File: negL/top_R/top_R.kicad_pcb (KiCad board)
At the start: 2 copper layers, 133.3 x 115.9 mm, 37 parts

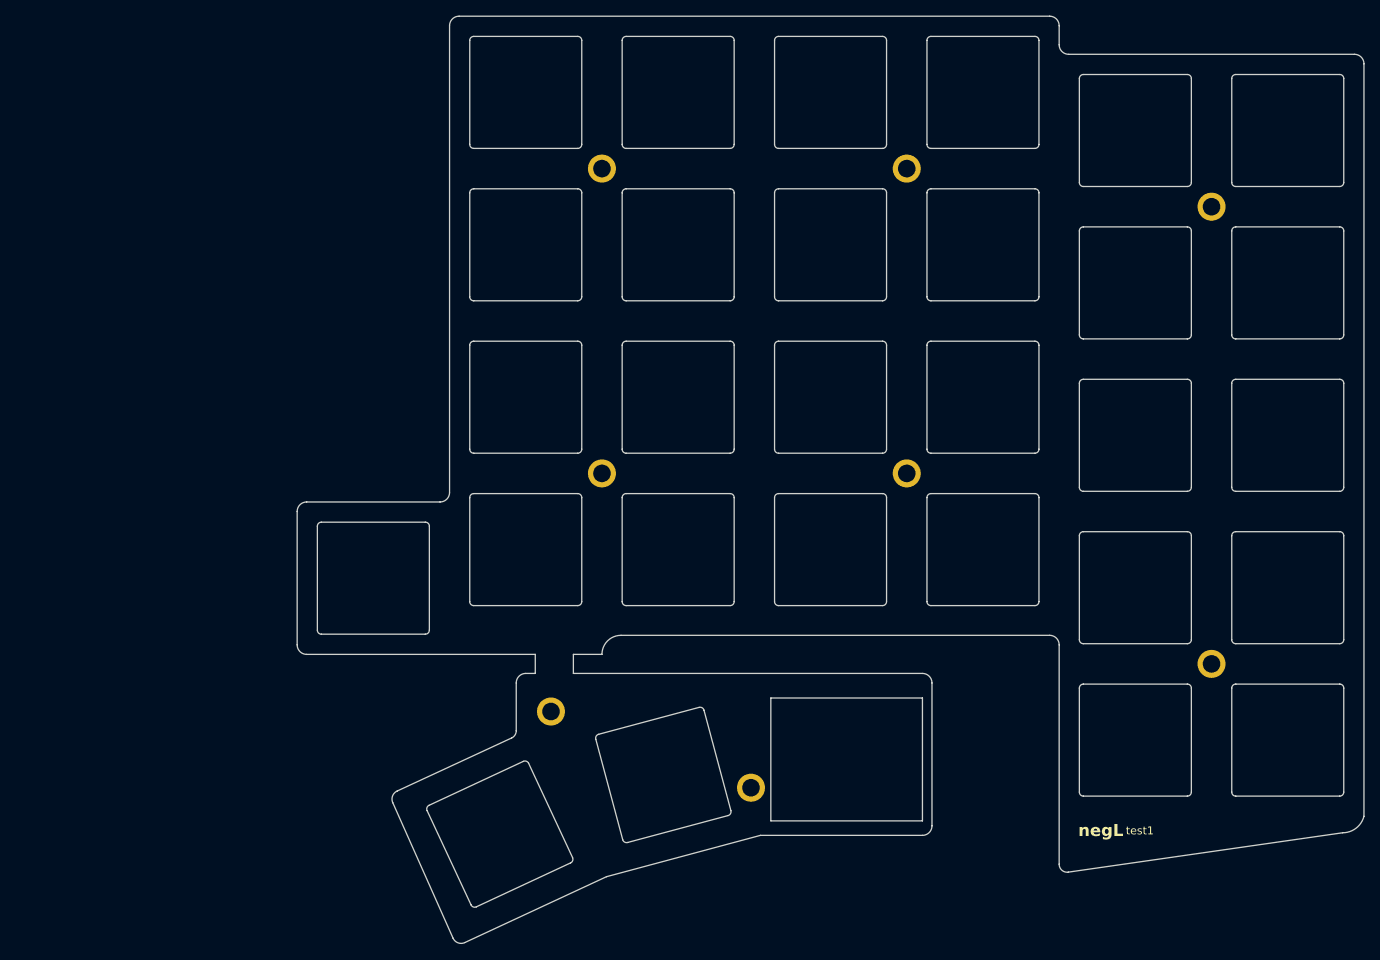
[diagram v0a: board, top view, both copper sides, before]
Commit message: add bottom
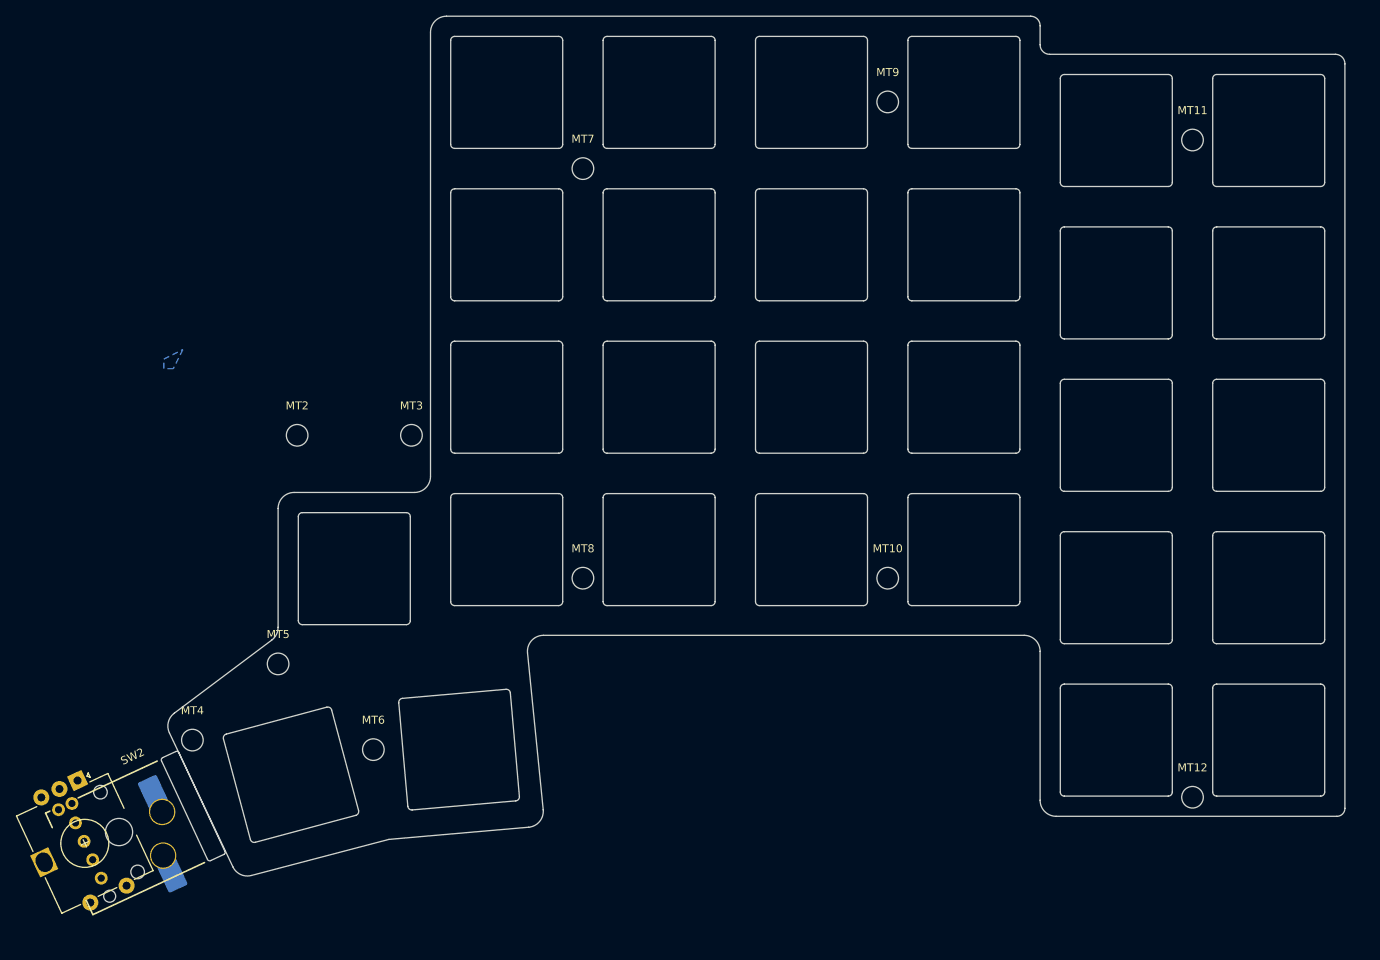
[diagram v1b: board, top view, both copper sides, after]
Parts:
- removed CH1, CH2: choc_v1_SW_HS, PCM_marbastlib-xp-plate-mx:Plate_MX_1u
- removed the MX20 at (120.3, 108.3)
- added MT12: MountingHole, MountingHole:MountingHole_2.7mm_M2.5, F.Cu at (203.6, 139.3)
- added MT2: MountingHole, MountingHole:MountingHole_2.7mm_M2.5, F.Cu at (91.7, 94.1)
- added MT3: MountingHole, MountingHole:MountingHole_2.7mm_M2.5, F.Cu at (106.0, 94.1)
- added MX20: MX_SW_HS, PCM_marbastlib-xp-plate-mx:Plate_MX_1u, B.Cu at (90.9, 136.5)
- added MX20: MX_SW_HS, PCM_marbastlib-xp-plate-mx:Plate_MX_1u, B.Cu at (111.9, 133.3)
- added MX20: MX_SW_HS, PCM_marbastlib-xp-plate-mx:Plate_MX_1u, B.Cu at (117.9, 108.3)
- added SW2: EVQWGD001_EC12, neg_footprints:choc_encoder, F.Cu at (72.0, 144.1)
- MT10, MT11, MT4, MT5, MT6, MT7, MT8, MT9: value M2_Top -> MountingHole; footprint neg_footprints:M2_Top -> MountingHole:MountingHole_2.7mm_M2.5
- moved MT6 78.0 mm to (101.2, 133.3)
- moved MT11 65.5 mm to (203.6, 57.1)
- moved MT8 65.3 mm to (127.4, 111.9)
- moved MT10 61.6 mm to (165.5, 111.9)
- moved MT5 61.1 mm to (89.3, 122.6)
- moved MT9 46.5 mm to (165.5, 52.4)
- moved MT4 45.0 mm to (78.6, 132.2)
- moved MT7 38.2 mm to (127.4, 60.7)
- moved MX19 2.66 mm to (98.8, 110.7)
- moved MX12 2.38 mm to (213.1, 75.0)
- moved MX18 2.38 mm to (213.1, 94.1)
- moved MX25 2.38 mm to (213.1, 113.1)
- moved MX27 2.38 mm to (213.1, 132.2)
- moved MX6 2.38 mm to (213.1, 56.0)
- moved MX1 2.38 mm to (117.9, 51.2)
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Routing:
- added copper zone on B.Cu, net Net-(BT1--)
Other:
- board size 133.3 x 115.9 mm -> 147.1 x 107.5 mm
- board text removed: "negL"
- board text removed: "test1"
